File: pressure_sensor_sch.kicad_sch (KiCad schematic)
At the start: 59 parts, among them J13 1053131104, U7 ADS131M06IPBS

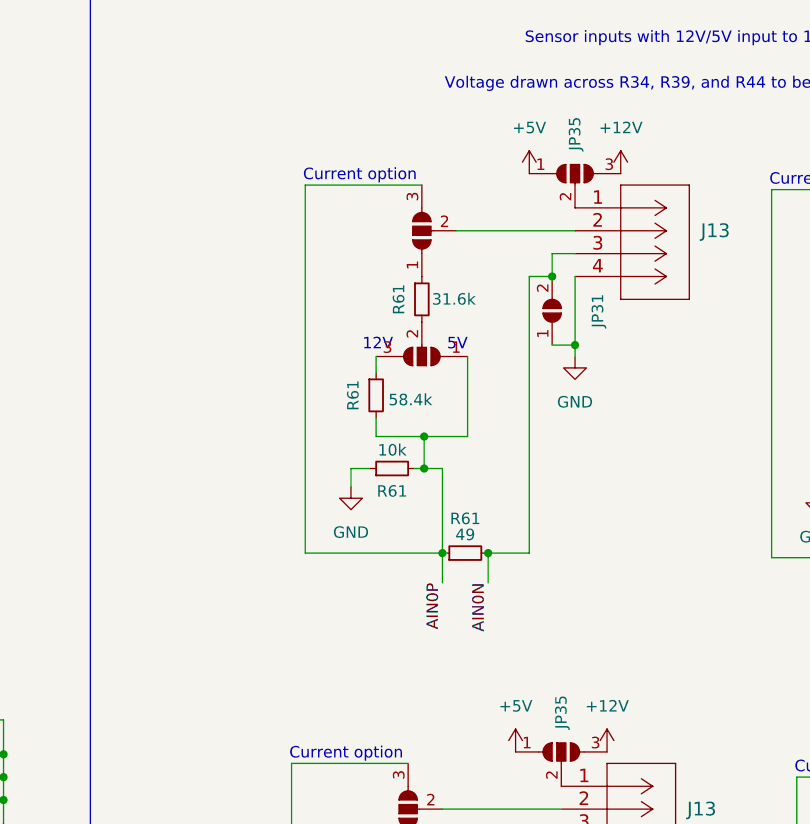
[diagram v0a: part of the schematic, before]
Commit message: commit
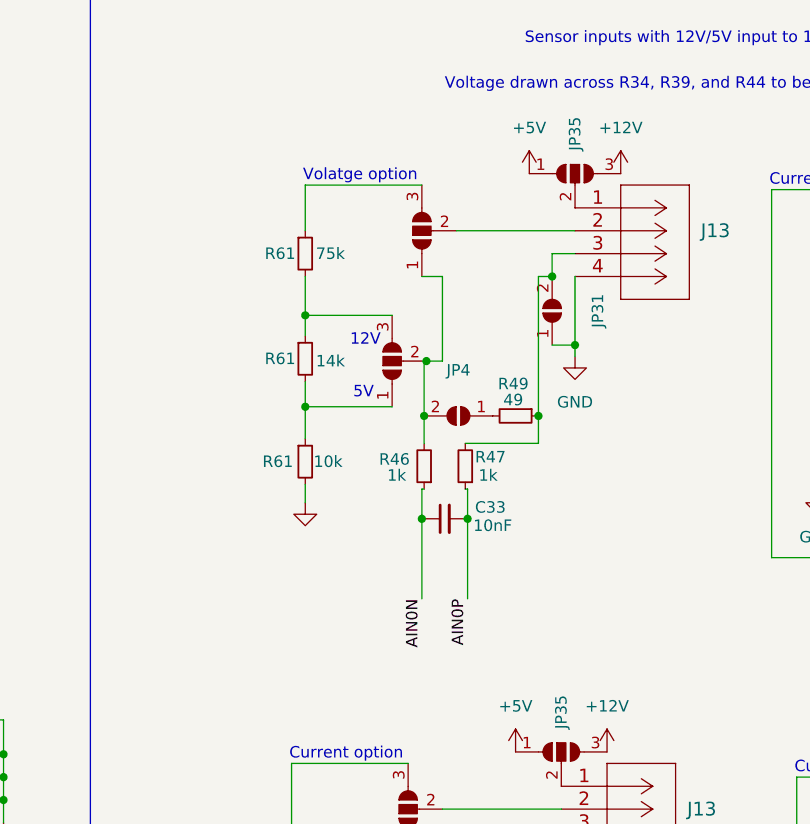
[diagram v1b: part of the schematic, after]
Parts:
- removed R61: 49, Resistor_SMD:R_0402_1005Metric, symbol Device:R_Small
- added C33: 10nF, Capacitor_SMD:C_0402_1005Metric, symbol Device:C_Small
- added JP4: SolderJumper_2_Open, iclr:SmallerSolderJP, symbol Jumper:SolderJumper_2_Open
- added R46, R47: 1k, Resistor_SMD:R_0402_1005Metric, symbol Device:R_Small
- added R49: 49, Resistor_SMD:R_0402_1005Metric, symbol Device:R_Small
- R61: value 58.4k -> 14k
- R61: value 31.6k -> 75k
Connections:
- net AIN0N: now also C33.1, R46.1; no longer J13.3, JP31.2 (B)
- net AIN0P: now also C33.2, R47.1; no longer JP39.1 (A), JP39.3 (B), R61.2, R61.2
- net GND: now also R61.2; no longer R61.1
- net at JP39.1 (A): now also JP39.2 (C), JP4.2 (B), R46.2; no longer R61.1
- net at JP39.3 (B), R61.1: now also R61.2
- new net: J13.3, JP31.2 (B), R47.2, R49.1
- new net: JP39.1 (A), R61.1, R61.2
- new net: JP39.3 (B), R61.1
- new net: JP4.1 (A), R49.2
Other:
- note added: "Volatge option"
- moved on the sheet: R61
